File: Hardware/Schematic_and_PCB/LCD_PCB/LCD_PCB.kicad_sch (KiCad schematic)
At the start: 14 parts, among them J1 LCD_display, J2 Conn_01x10, SW1 Button_down, SW2 Button_up, SW3 Button_ok, SW4 Button_back, SW5 SW_Push

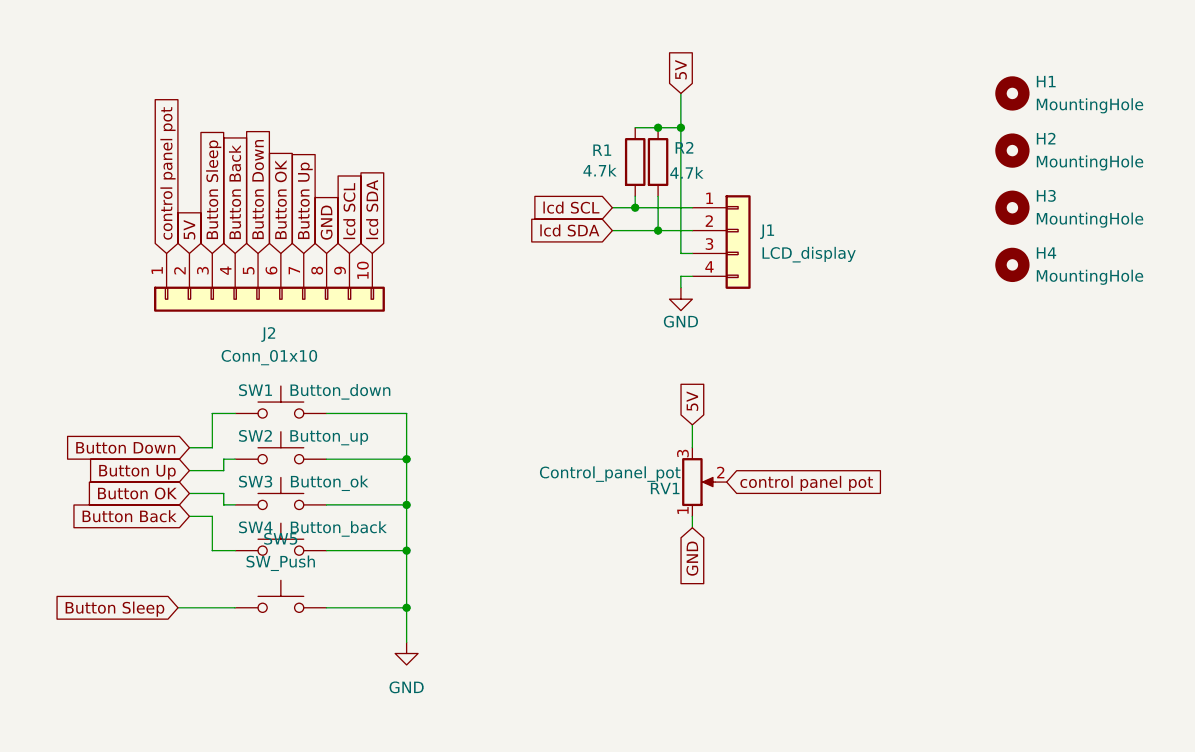
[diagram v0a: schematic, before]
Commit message: Code update for room 3
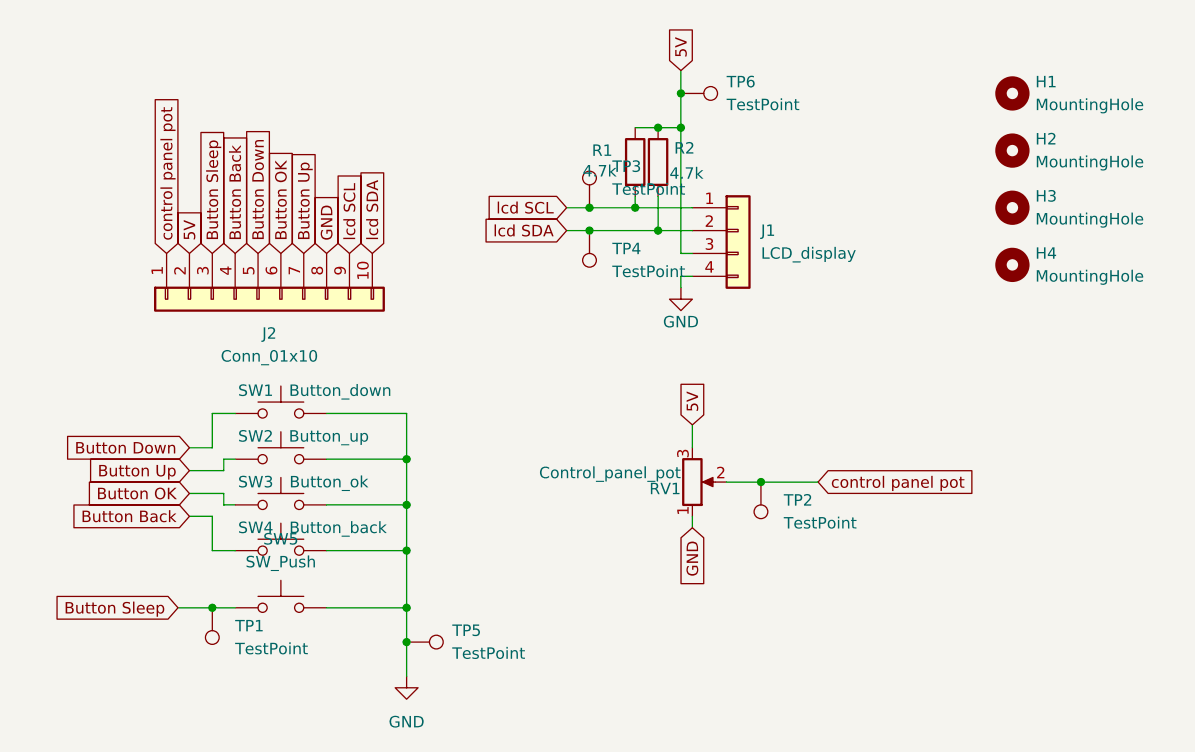
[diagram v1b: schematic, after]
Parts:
- added TP1, TP2, TP3, TP4, TP5, TP6: TestPoint, TestPoint:TestPoint_Pad_1.5x1.5mm, symbol Connector:TestPoint
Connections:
- net 5V: now also TP6.1
- net Button Sleep: now also TP1.1
- net GND: now also TP5.1
- net control panel pot: now also TP2.1
- net lcd SCL: now also TP3.1
- net lcd SDA: now also TP4.1
